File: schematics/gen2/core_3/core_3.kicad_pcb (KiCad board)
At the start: 2 copper layers, 84.3 x 8.4 mm, 7 parts

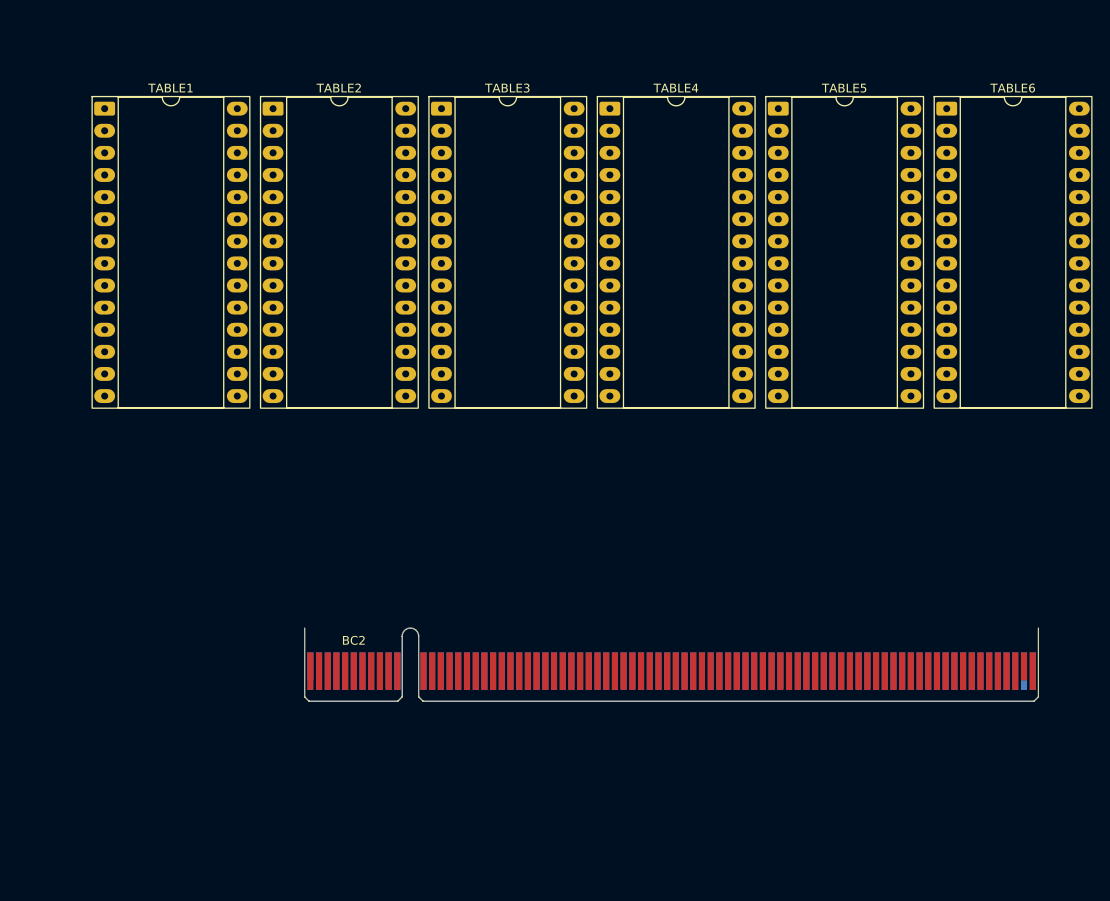
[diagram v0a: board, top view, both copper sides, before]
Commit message: Add core 3
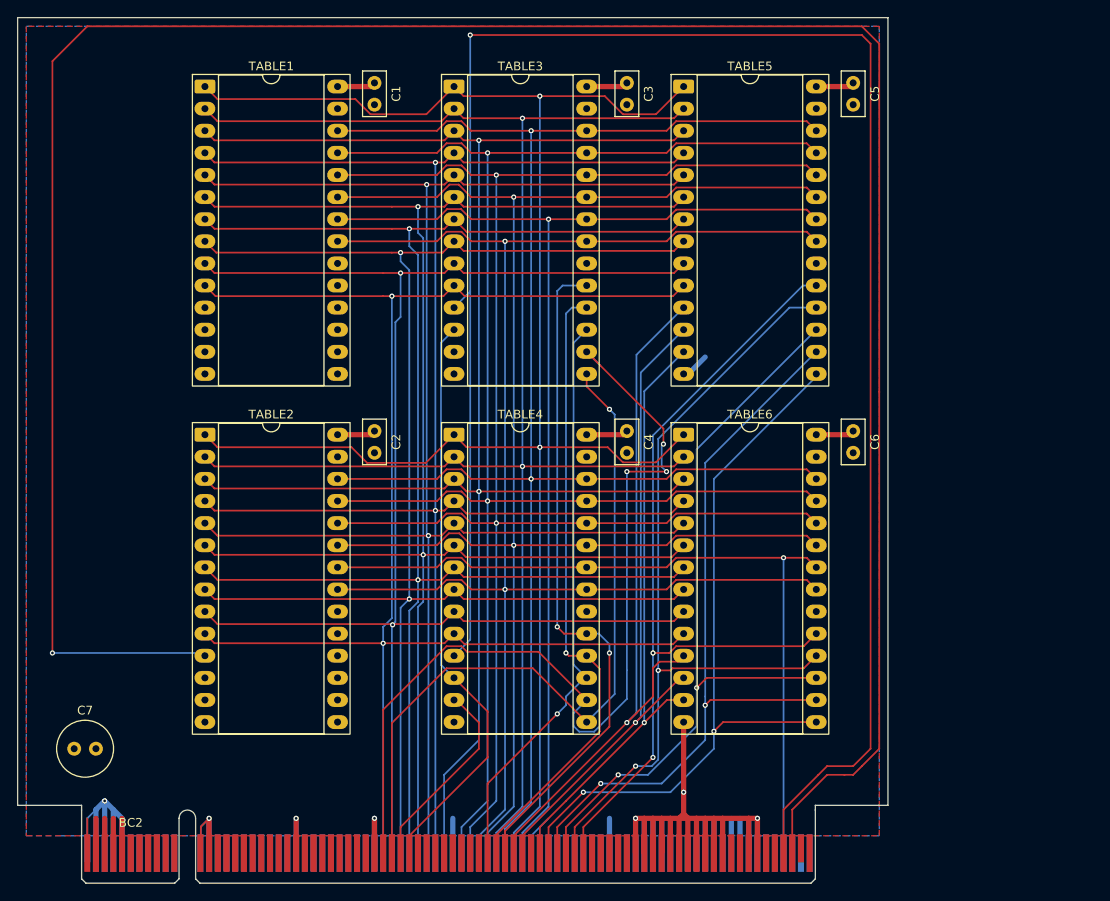
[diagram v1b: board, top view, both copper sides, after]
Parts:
- added C1: C, Capacitor_THT:C_Disc_D5.0mm_W2.5mm_P2.50mm, F.Cu at (94.0, 60.5)
- added C2: C, Capacitor_THT:C_Disc_D5.0mm_W2.5mm_P2.50mm, F.Cu at (94.0, 100.5)
- added C3: C, Capacitor_THT:C_Disc_D5.0mm_W2.5mm_P2.50mm, F.Cu at (123.0, 60.5)
- added C4: C, Capacitor_THT:C_Disc_D5.0mm_W2.5mm_P2.50mm, F.Cu at (123.0, 100.5)
- added C5: C, Capacitor_THT:C_Disc_D5.0mm_W2.5mm_P2.50mm, F.Cu at (149.0, 60.5)
- added C6: C, Capacitor_THT:C_Disc_D5.0mm_W2.5mm_P2.50mm, F.Cu at (149.0, 100.5)
- added C7: C, Capacitor_THT:C_Radial_D6.3mm_H5.0mm_P2.50mm, F.Cu at (59.5, 137.0)
- moved TABLE6 48.1 mm to (129.5, 100.9)
- moved TABLE4 41.5 mm to (103.1, 100.9)
- moved TABLE2 38.3 mm to (74.5, 100.9)
- moved BC2 33.1 mm to (61.0, 149.0)
- moved TABLE1 11.8 mm to (74.5, 60.9)
- moved TABLE5 11.2 mm to (129.5, 60.9)
- moved TABLE3 2.92 mm to (103.1, 60.9)
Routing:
- net Net-(BC2-R4): track 0.00 -> 282.0 mm, vias 0 -> 1
- net Net-(BC2-L4): track 0.00 -> 220.0 mm, vias 0 -> 1
- net /STATE14: track 0.00 -> 208.8 mm, vias 0 -> 2
- net /STATE12: track 0.00 -> 199.6 mm, vias 0 -> 2
- net /STATE13: track 0.00 -> 197.9 mm, vias 0 -> 2
- net /STATE7: track 0.00 -> 197.5 mm, vias 0 -> 2
- net /STATE8: track 0.00 -> 195.4 mm, vias 0 -> 2
- net /STATE6: track 0.00 -> 193.3 mm, vias 0 -> 2
- net /STATE9: track 0.00 -> 192.8 mm, vias 0 -> 2
- net /STATE5: track 0.00 -> 190.9 mm, vias 0 -> 2
- net /STATE11: track 0.00 -> 190.8 mm, vias 0 -> 2
- net /STATE4: track 0.00 -> 188.7 mm, vias 0 -> 2
- net /STATE3: track 0.00 -> 186.8 mm, vias 0 -> 2
- net /STATE10: track 0.00 -> 185.2 mm, vias 0 -> 2
- net /STATE2: track 0.00 -> 183.6 mm, vias 0 -> 2
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- added copper zone on B.Cu, net GND
- added copper zone on F.Cu, net VCC
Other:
- board size 84.3 x 8.4 mm -> 100 x 91.1 mm
